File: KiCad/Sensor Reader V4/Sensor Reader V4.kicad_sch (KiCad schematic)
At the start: 66 parts, among them IC1 TLV76733DGNR, IC2 ESP32-C3-WROOM-02-H4, J10 L_I/B1_Out, J11 B1_Net/B2_In, J12 B2_Net/B2_Out, J13 AIN_4, J14 AIN_5, J15 5V_Input, J16 3.3V_Output, J2 UJ20-C-H-G-MSMT-2B-P16-TR, J6 Exposed_UART, J7 Batt1_V, J8 Batt2_V, J9 M_OUT/B1_In, SW1 BOOT_Btn, SW2 EN_Btn, U3 ADS8688

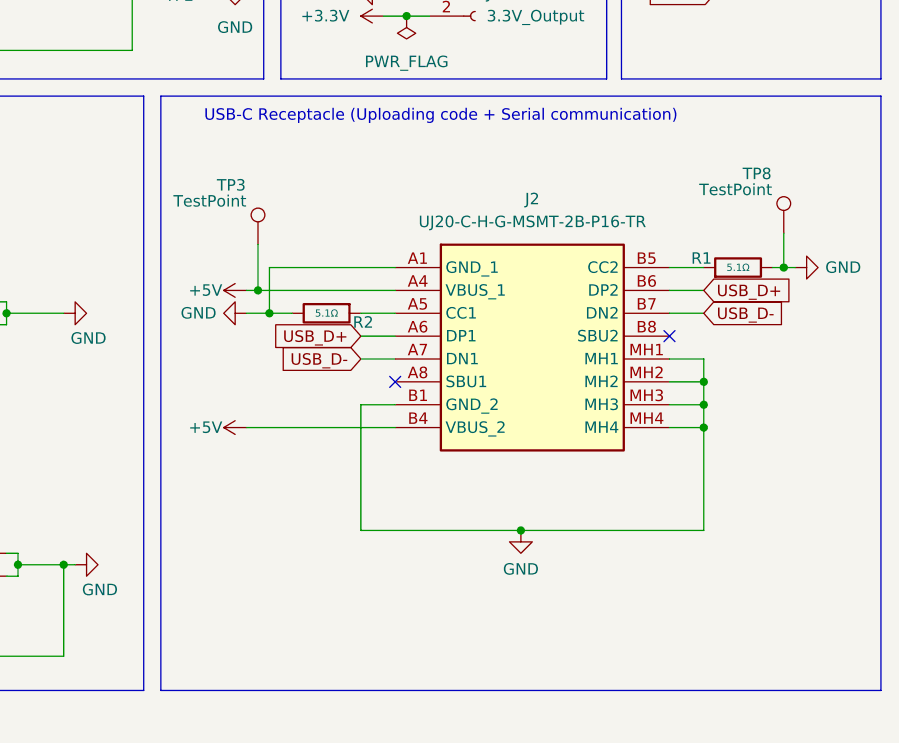
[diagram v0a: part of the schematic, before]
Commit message: KICAD pcb
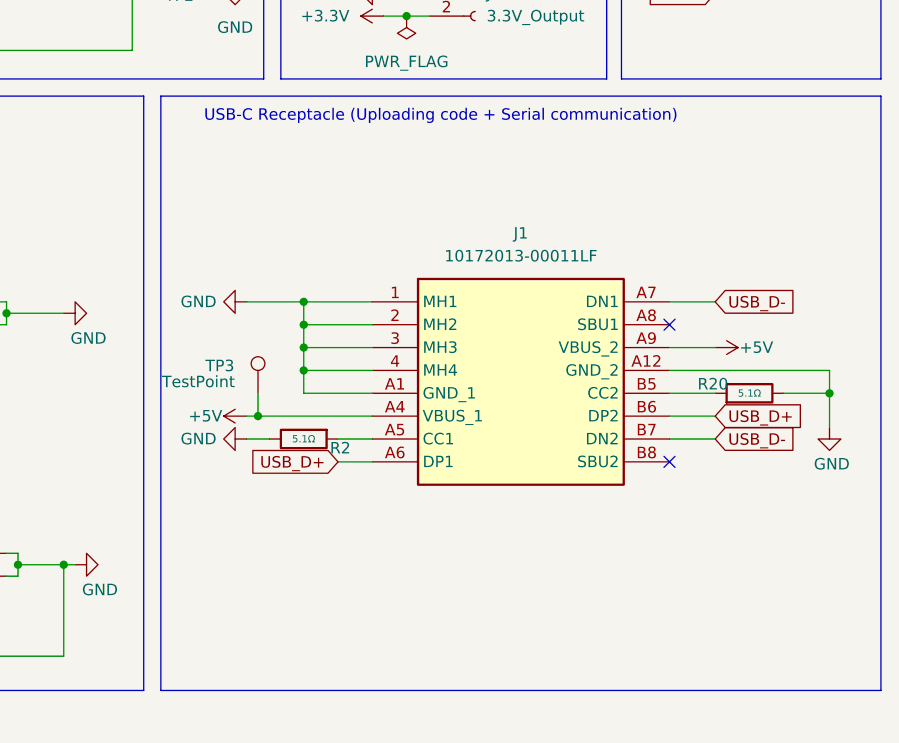
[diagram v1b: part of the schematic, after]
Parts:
- removed J2: UJ20-C-H-G-MSMT-2B-P16-TR, SamacSys_Parts:UJ20CHGMSMT2BP16TR, symbol SamacSys_Parts:UJ20-C-H-G-MSMT-2B-P16-TR
- removed R1: 5.1Ω, Resistor_SMD:R_0603_1608Metric_Pad0.98x0.95mm_HandSolder, symbol PCM_JLCPCB-Resistors:0603,5.1Ω
- removed TP8: TestPoint, TestPoint:TestPoint_Pad_D1.0mm, symbol Connector:TestPoint
- added J1: 10172013-00011LF, 1017201300011LF, symbol SamacSys_Parts:10172013-00011LF
- added R20: 5.1Ω, Resistor_SMD:R_0603_1608Metric_Pad0.98x0.95mm_HandSolder, symbol PCM_JLCPCB-Resistors:0603,5.1Ω
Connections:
- net +5V: now also J1.A4 (VBUS_1), J1.A9 (VBUS_2)
- net GND: now also J1.1 (MH1), J1.2 (MH2), J1.3 (MH3), J1.4 (MH4), J1.A1 (GND_1), J1.A12 (GND_2), R20.2
- net USB_D+: now also J1.A6 (DP1), J1.B6 (DP2)
- net USB_D-: now also J1.A7 (DN1), J1.B7 (DN2)
- net at R2.1: now also J1.A5 (CC1)
- new net: J1.B5 (CC2), R20.1
